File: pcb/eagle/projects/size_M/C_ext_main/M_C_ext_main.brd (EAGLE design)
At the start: 18 parts, among them P1 TPB1,27, U1 CP2104-F03-GM

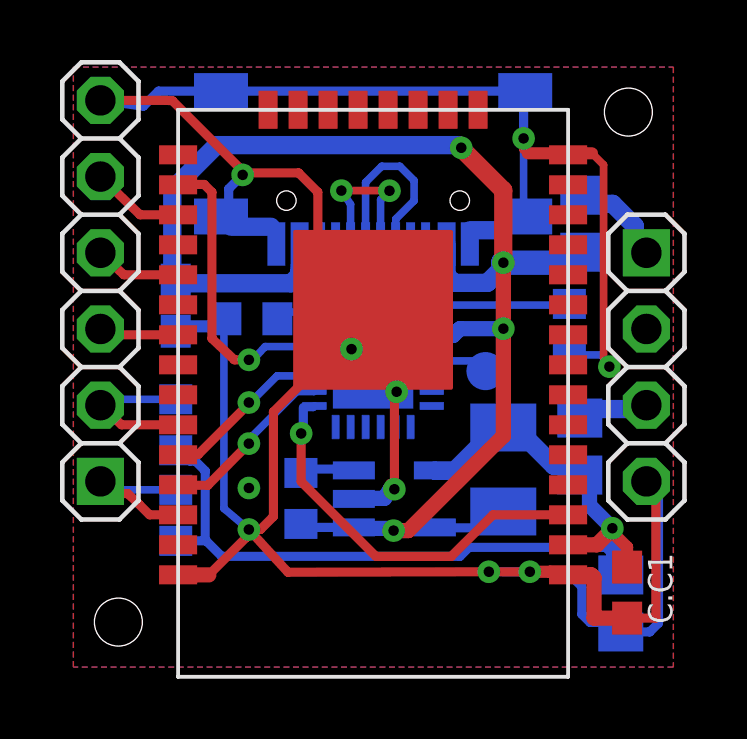
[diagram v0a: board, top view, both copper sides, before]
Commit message: PCB v4
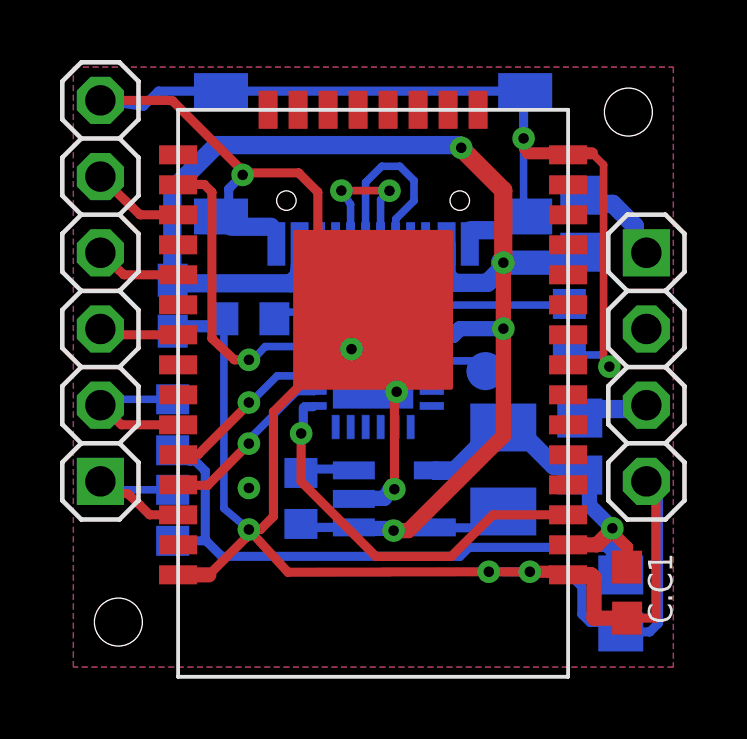
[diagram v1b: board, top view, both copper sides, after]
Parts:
- moved C.C5 0.10 mm to (3.81, 12.5)
- moved C.R1 0.10 mm to (3.81, 5.56)
- moved C.R2 0.10 mm to (3.81, 8.58)
- moved C.R6 0.10 mm to (6.35, 12.1)
